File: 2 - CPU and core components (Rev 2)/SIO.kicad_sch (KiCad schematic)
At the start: 23 parts

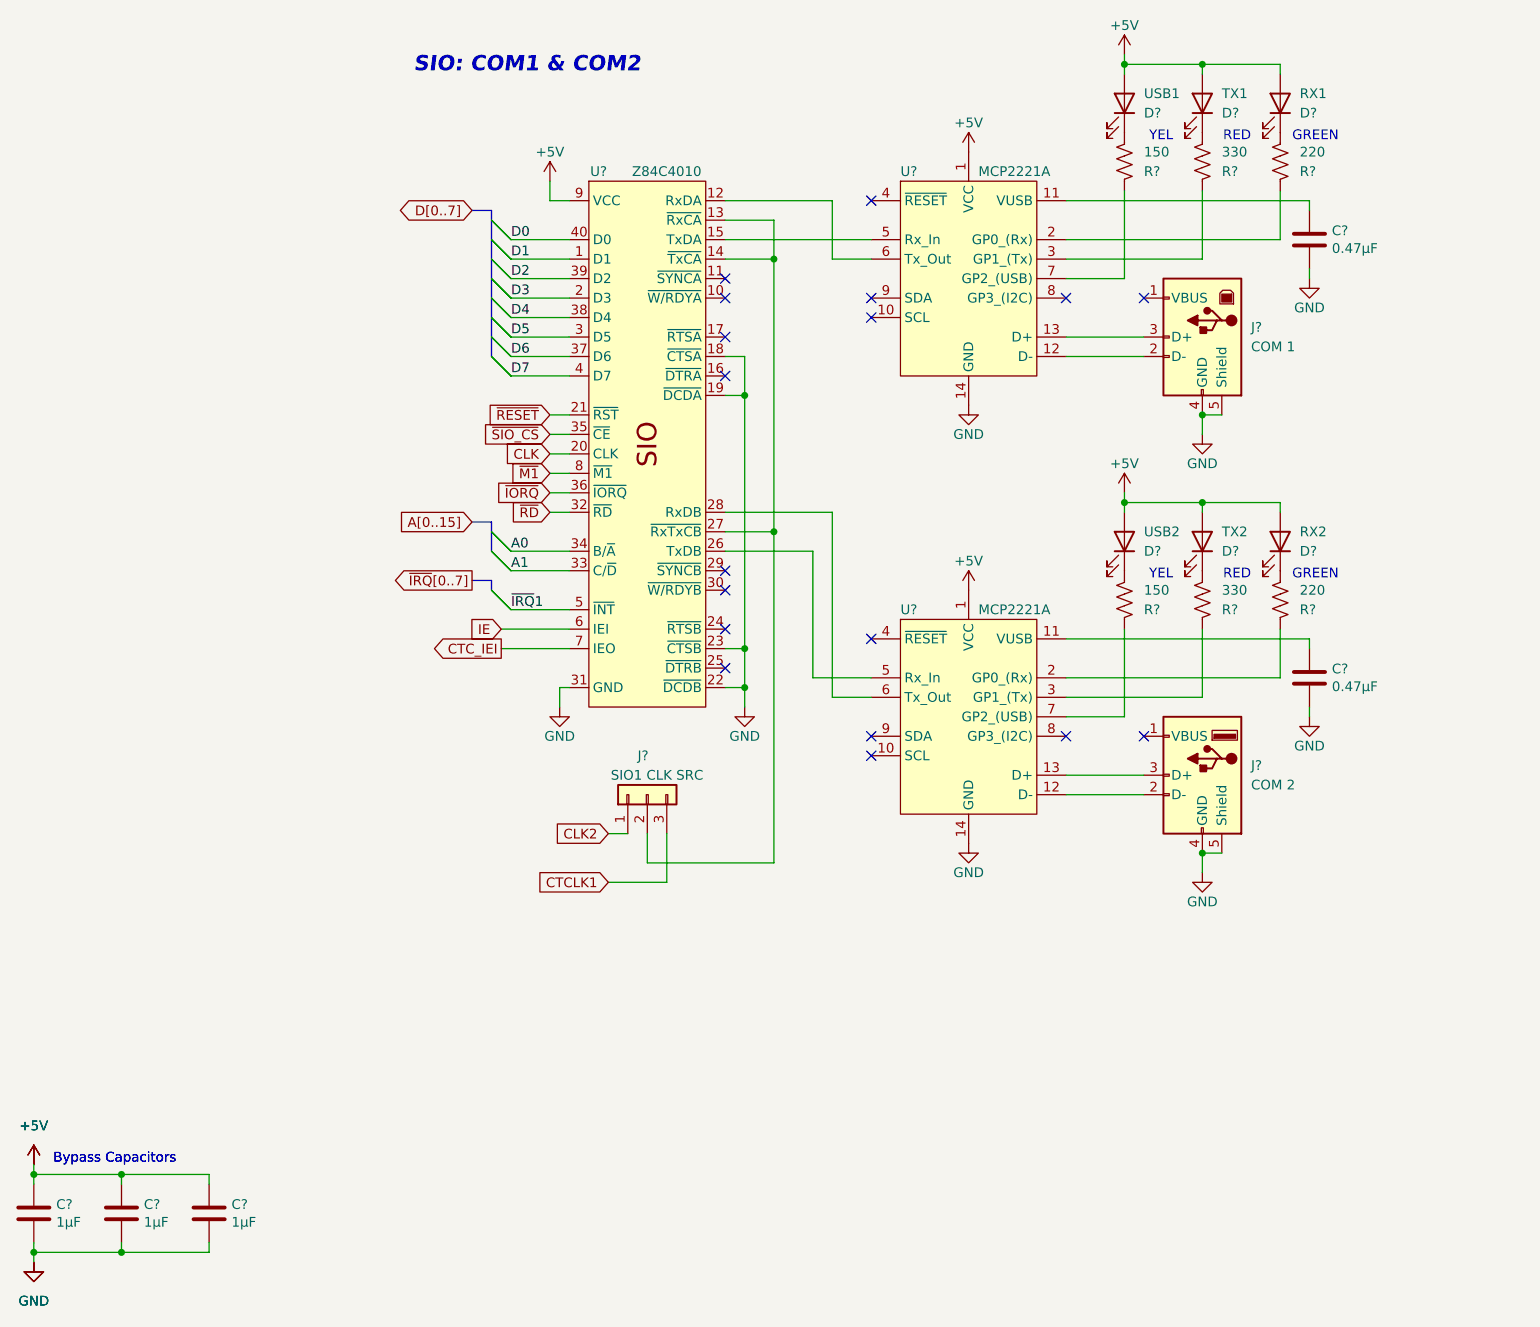
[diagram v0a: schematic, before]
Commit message: Finished component placement, currently routing.
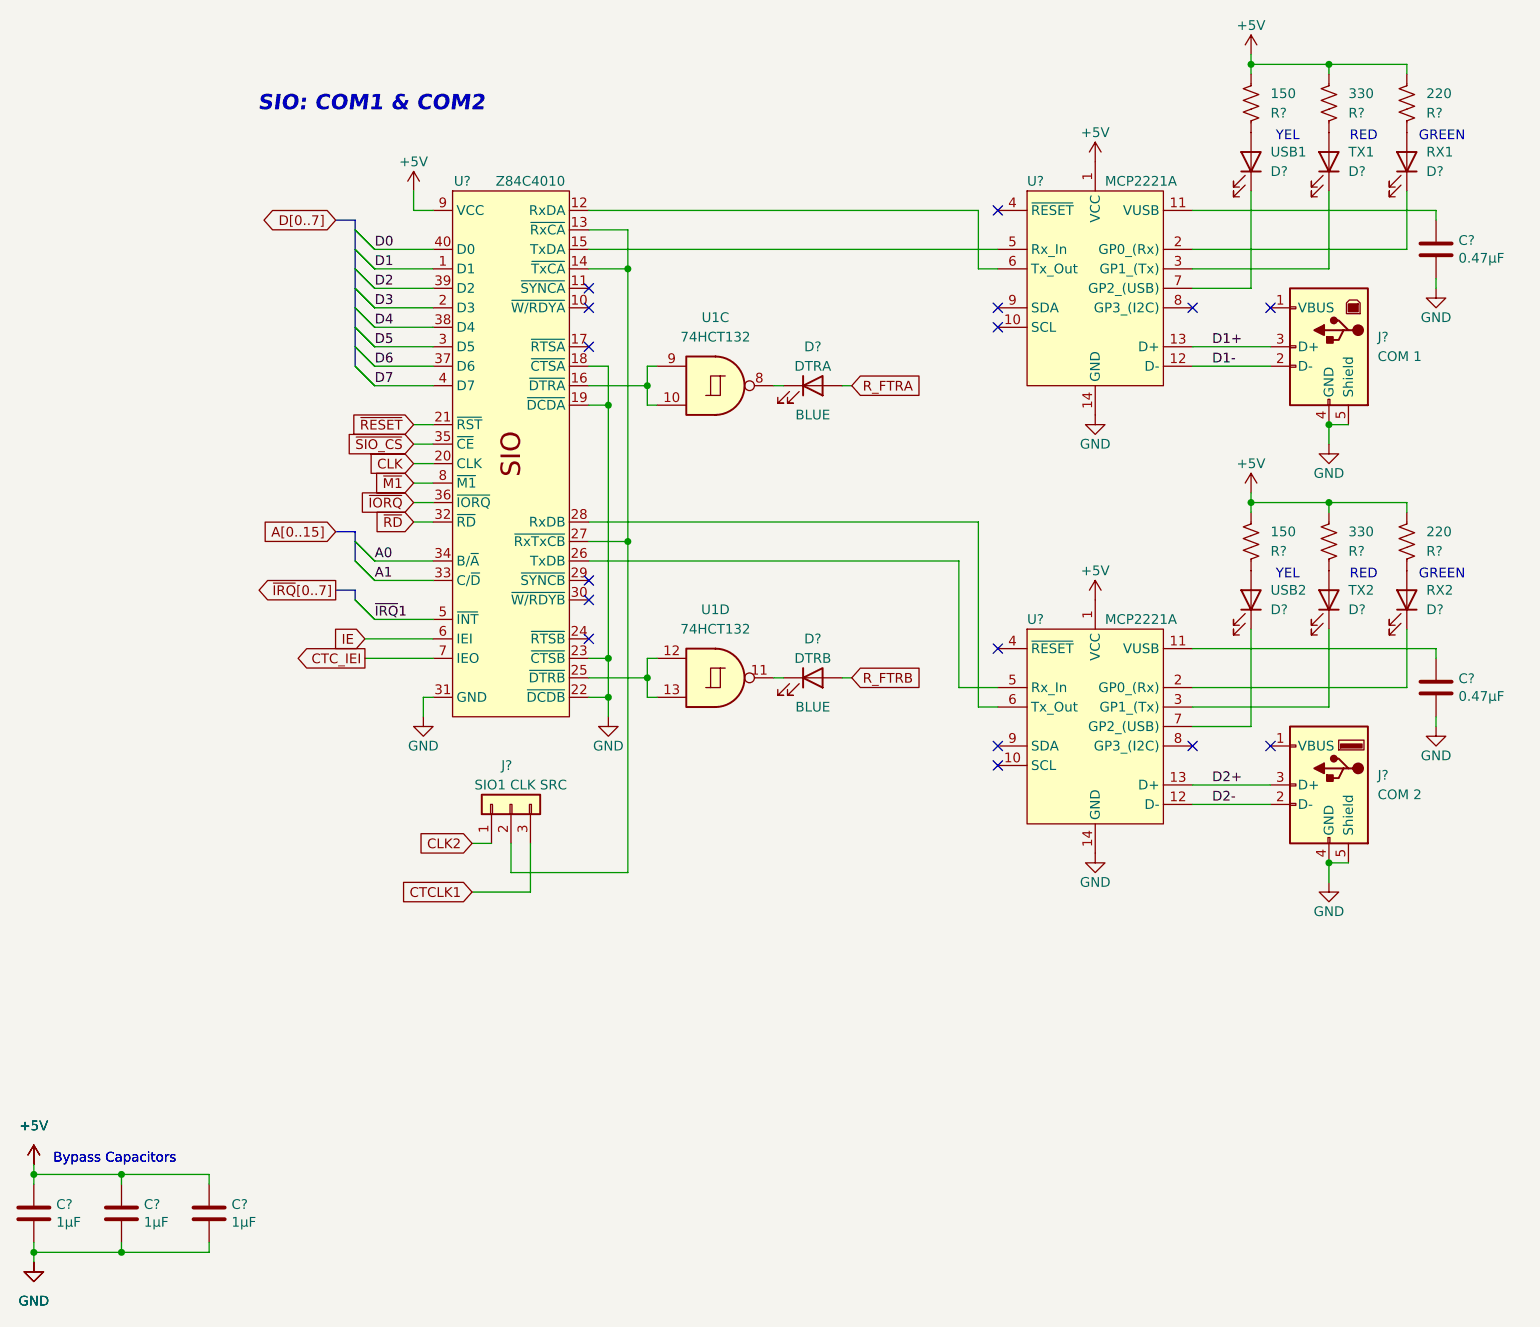
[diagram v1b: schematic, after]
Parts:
- added D?: DTRB, LED_THT:LED_D3.0mm_Horizontal_O1.27mm_Z2.0mm_Clear, symbol Device:LED
- added D?: DTRA, LED_THT:LED_D3.0mm_Horizontal_O1.27mm_Z2.0mm_Clear, symbol Device:LED
- added U1: 74HCT132, Package_DIP:DIP-14_W7.62mm_Socket, symbol 74xx:74LS132
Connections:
- net +5V: now also R?.2, R?.2, R?.2, R?.2, R?.2, R?.2; no longer D?.2 (A), D?.2 (A), D?.2 (A), D?.2 (A), D?.2 (A), D?.2 (A)
- net at R?.1: now also D?.2 (A); no longer U?.2 (GP0_(Rx))
- net at D?.1 (K): now also U?.2 (GP0_(Rx)); no longer R?.2
- net D1-: now reaches J?.2 (D-), U?.12 (D-)
- net D1+: now reaches J?.3 (D+), U?.13 (D+)
- net at U?.3 (GP1_(Tx)): now also D?.1 (K); no longer R?.1 (x2)
- net at U?.7 (GP2_(USB)): now also D?.1 (K); no longer R?.1
- net at D?.1 (K): now also U?.7 (GP2_(USB)); no longer R?.2
- net D2-: now reaches J?.2 (D-), U?.12 (D-)
- net D2+: now reaches J?.3 (D+), U?.13 (D+)
- net at U?.2 (GP0_(Rx)): now also D?.1 (K); no longer R?.1
- net at R?.1: now also D?.2 (A); no longer U?.7 (GP2_(USB))
- net at U?.16 (~{DTRA}): now also U1.10, U1.9
- net at U?.25 (~{DTRB}): now also U1.12, U1.13
- new net: D?.1 (K), U1.11
- new net: D?.1 (K), U1.8
- new net: D?.2 (A), R?.1 (x4)
- new net R_FTRA: D?.2 (A)
- new net R_FTRB: D?.2 (A)
- no-connect marks 18 -> 16
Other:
- moved on the sheet: C?, D?, J?, R?, U?
